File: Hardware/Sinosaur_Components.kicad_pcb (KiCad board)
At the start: 4 copper layers, 60 x 100 mm, 83 parts, among them J1 Conn_01x12_Male, J2 Conn_01x12_Male, J3 Conn_01x16_Male, J4 Conn_01x16_Male, J5 SWD_Header, J6 Eurorack_16_pin_power, J7 UART_Test_Pins, J8 USB_B_Micro, Q1 MMBT3904, Q2 MMBT3904, U1 STM32G473V, U2 STF202-22T1G, U3 TL074, U4 TL074, U5 LT1117-3.3, Y1 8MHz 20pF

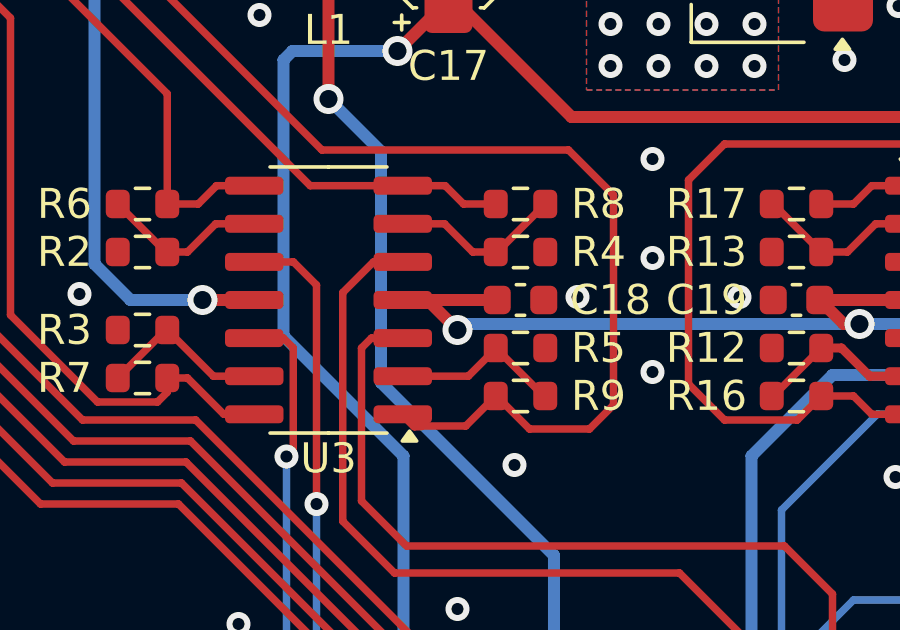
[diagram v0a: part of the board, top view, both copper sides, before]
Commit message: Gerber production for v1
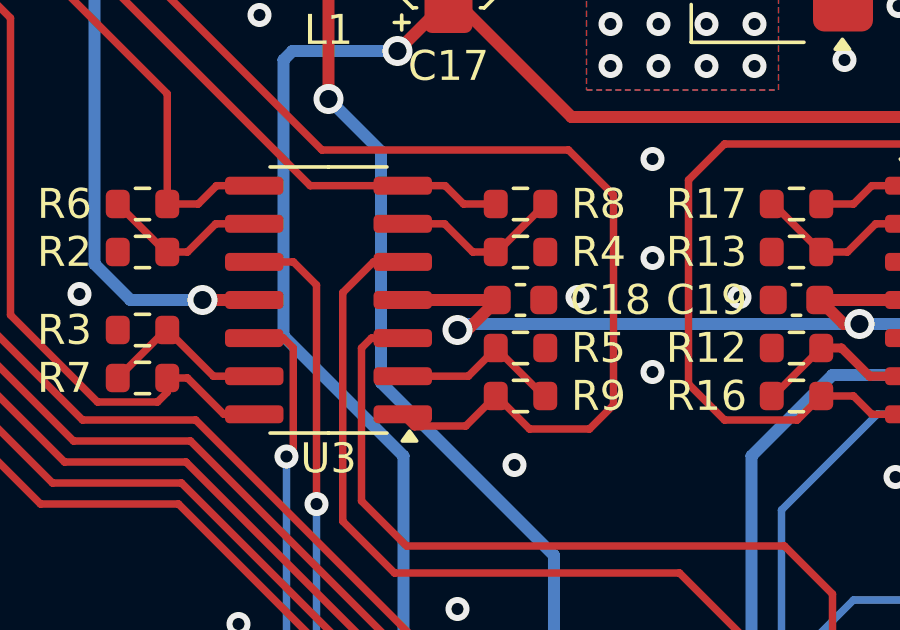
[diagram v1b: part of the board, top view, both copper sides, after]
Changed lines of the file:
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@@
-	)
-	(segment
-		(start 122.3 79)
-		(end 121.475 79)
-		(width 0.4)
-		(layer "F.Cu")
-		(net 5)
 	)
 	(segment
 		(start 147 56.65)
 		(end 150.85 56.65)
-		(width 0.4)
-		(layer "F.Cu")
-		(net 5)
-	)
-	(segment
-		(start 121.8625 79)
-		(end 124.625 79)
 		(width 0.4)
 		(layer "F.Cu")
@@
 	)
 	(segment
+		(start 123.3 80)
+		(end 123.625 80)
+		(width 0.4)
+		(layer "F.Cu")
+		(net 5)
+	)
+	(segment
 		(start 151 57.7)
 		(end 141.45 67.25)
@@
 		(start 136.175 79.8)
 		(end 135.375 79)
-		(width 0.4)
-		(layer "F.Cu")
-		(net 5)
-	)
-	(segment
-		(start 123.3 80)
-		(end 122.3 79)
 		(width 0.4)
 		(layer "F.Cu")
@@
 	)
 	(segment
+		(start 123.625 80)
+		(end 124.625 79)
+		(width 0.4)
+		(layer "F.Cu")
+		(net 5)
+	)
+	(segment
 		(start 141.45 68.55)
 		(end 139.925 68.55)
 		(width 0.4)
 		(layer "F.Cu")
+		(net 5)
+	)
+	(segment
+		(start 124.625 79)
+		(end 121.475 79)
+		(width 0.4)
+		(layer "F.Cu")
